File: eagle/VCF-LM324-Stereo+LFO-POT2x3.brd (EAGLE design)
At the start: 55.9 x 58.4 mm, 50 parts, among them IC1 LM324, J1 A_IN, J2 A_OUT, J3 CONN-2P2P/H

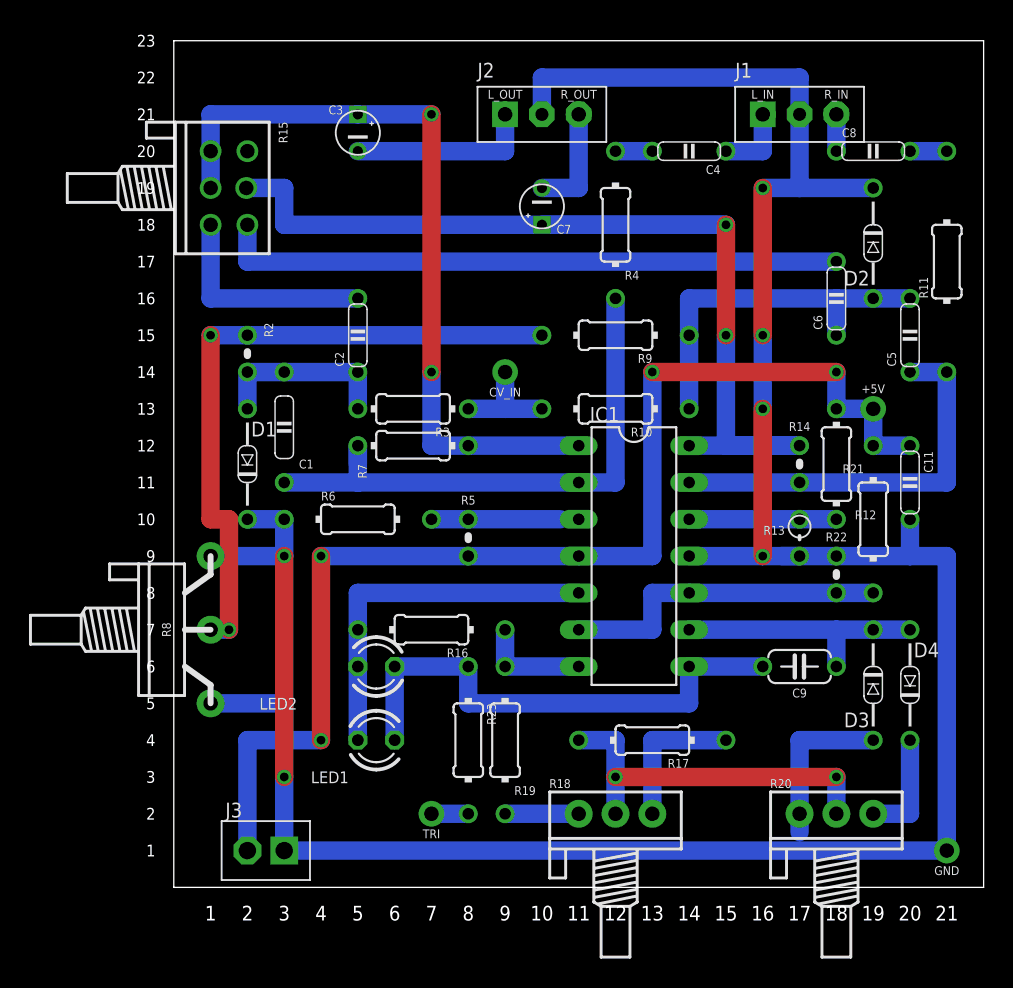
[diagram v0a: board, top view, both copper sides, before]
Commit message: ...
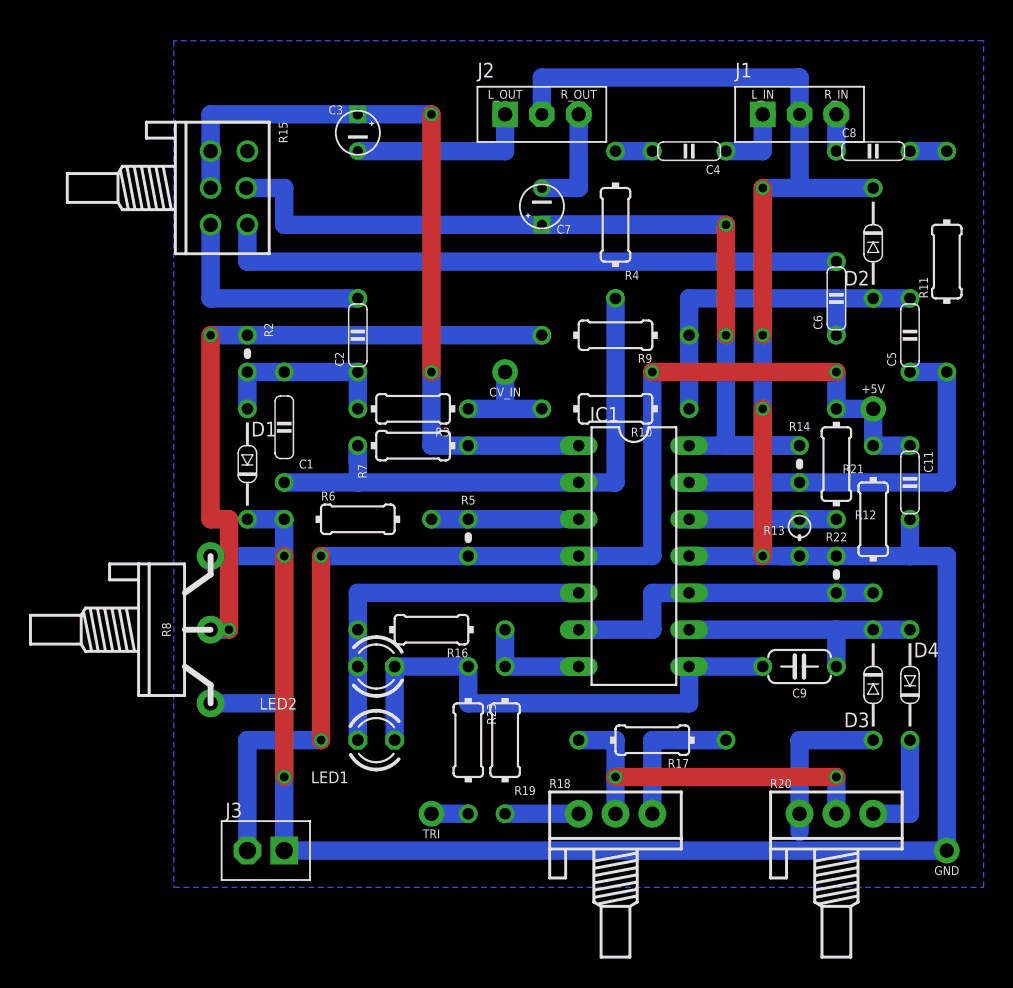
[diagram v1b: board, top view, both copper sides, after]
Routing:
- added copper zone on layer 16, net GND
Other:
- board outline removed
